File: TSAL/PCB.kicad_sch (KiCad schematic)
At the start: 44 parts, among them J1 TE 770966-2, J2 JST B04B-XASK, Q1 IRLZ44N, Q2 MMBT3904, Q3 IRLZ44N, U1 TL431D, U2 LMV331, U3 VRB1205YMD-6WR3, U4 LTV-817S, U5 LM555xN

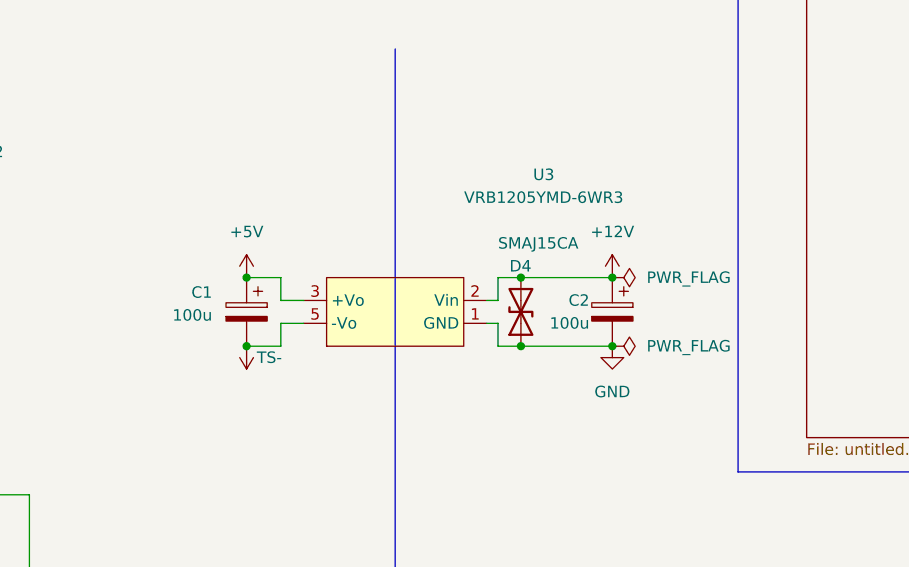
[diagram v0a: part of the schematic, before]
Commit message: TSAL W/ updated DC-DC + Meme
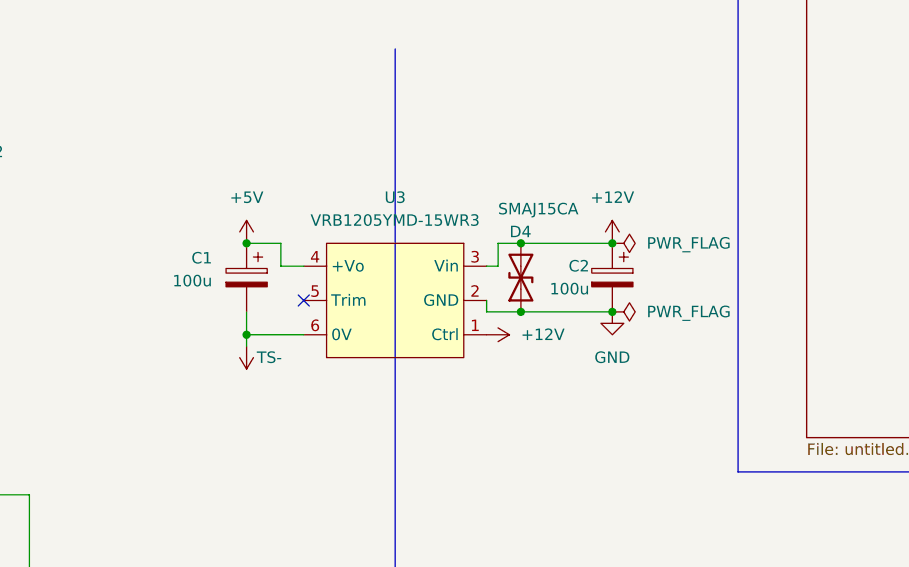
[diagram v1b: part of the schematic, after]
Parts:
- removed U3: VRB1205YMD-6WR3, VRB1205YMD-6WR3:VRB1205YMD-6WR3, symbol VRB1205YMD-6WR3:VRB1205YMD-6WR3
- added U3: VRB1205YMD-15WR3, VRB1205YMD-6WR3:VRB1205YMD-15WR3, symbol VRB1205YMD-6WR3:VRB1205YMD-15WR3
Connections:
- net +12V: now also U3.1 (Ctrl), U3.3 (Vin)
- net +5V: now also U3.4 (+Vo)
- net GND: now also U3.2 (GND)
- net TS-: now also U3.6 (0V)
- no-connect marks 0 -> 1
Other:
- moved on the sheet: C1, C2, D4
